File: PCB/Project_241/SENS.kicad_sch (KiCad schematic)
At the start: 15 parts, among them J2 Wind_Hall, J5 Rain_Hall, U3 LM393, U5 HDC1080

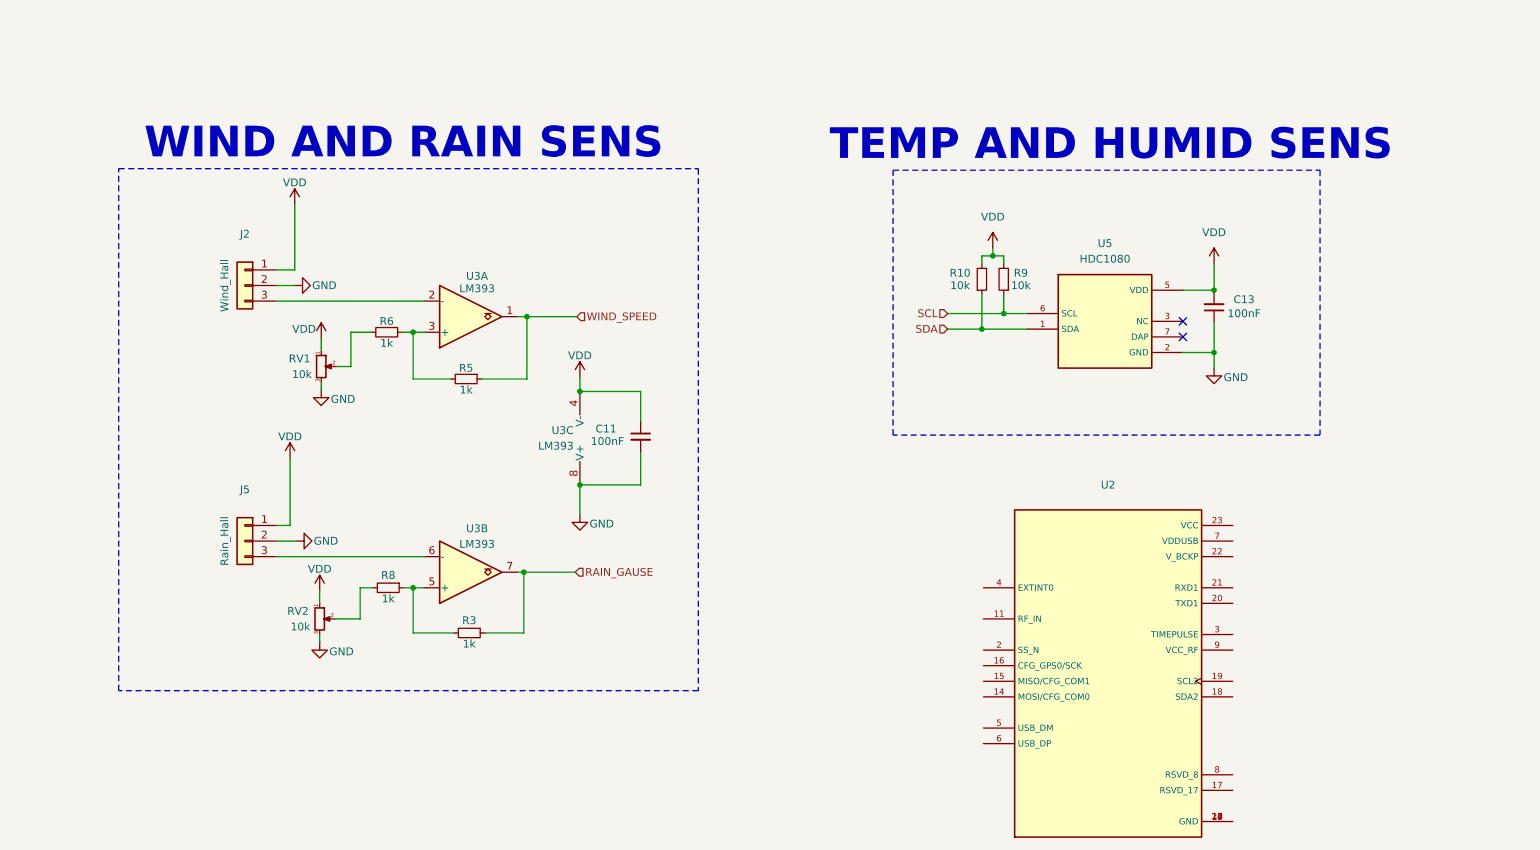
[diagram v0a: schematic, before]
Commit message: update gerber
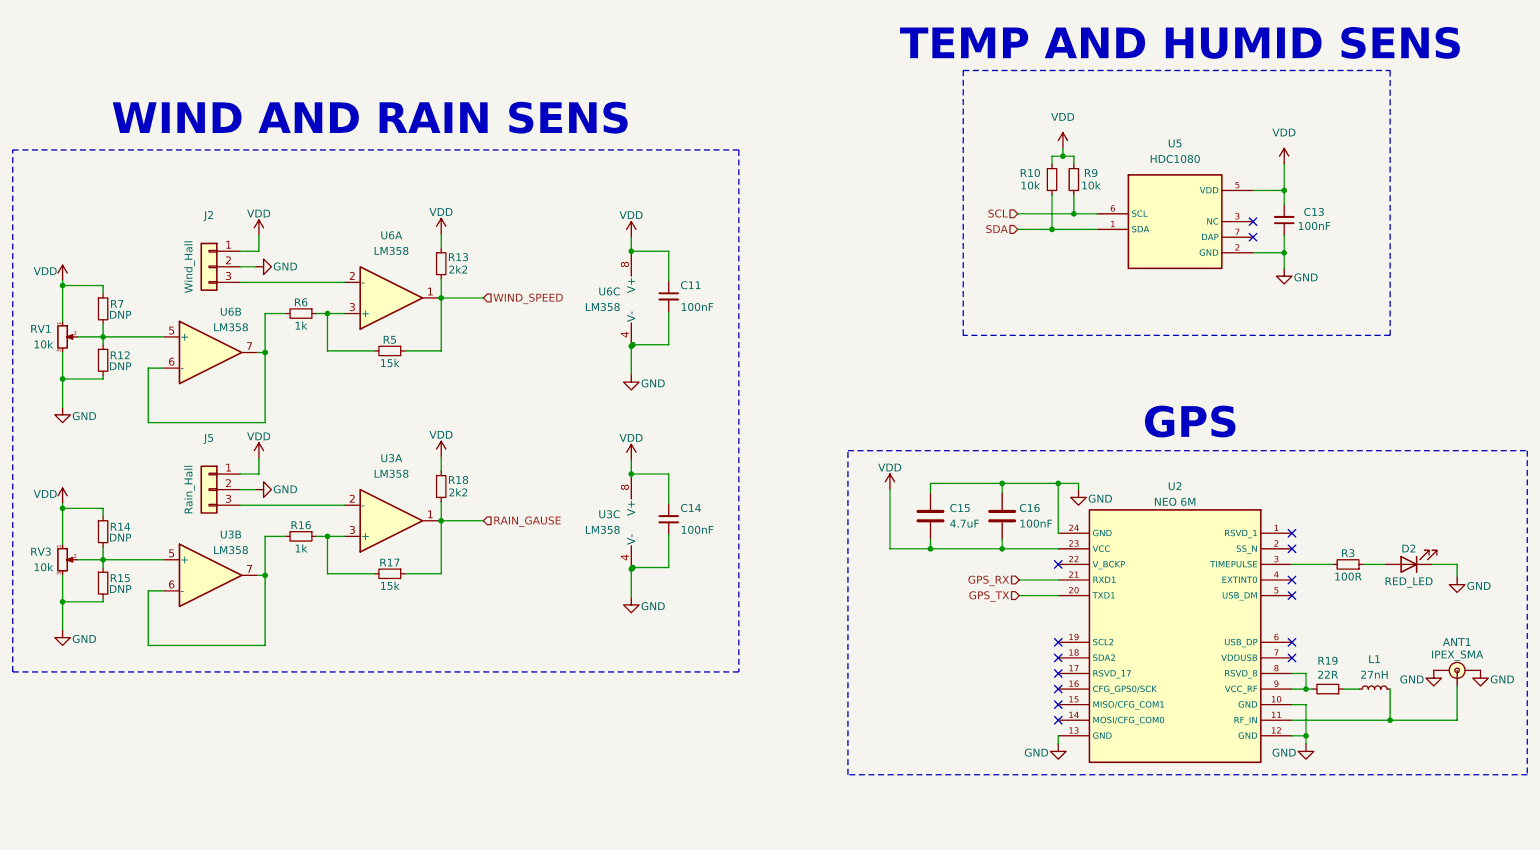
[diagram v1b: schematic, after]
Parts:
- removed R8: 1k, Resistor_SMD:R_0603_1608Metric, symbol Device:R_Small
- removed RV2: 10k, Resistor_SMD:R_0603_1608Metric, symbol Device:R_Potentiometer_Small
- removed U3: LM393, Package_SO:SO-8_3.9x4.9mm_P1.27mm, symbol Comparator:LM393
- added ANT1: IPEX_SMA, project241_footprint:ANT_SMA_3PIN, symbol project241_sym:IPEX_ANT
- added C14: 100nF, Capacitor_SMD:C_0603_1608Metric, symbol Device:C_Small
- added C15: 4.7uF, Capacitor_SMD:C_0603_1608Metric, symbol Device:C
- added C16: 100nF, Capacitor_SMD:C_0603_1608Metric, symbol Device:C
- added D2: RED_LED, LED_SMD:LED_0603_1608Metric, symbol Device:LED
- added L1: 27nH, Inductor_SMD:L_0603_1608Metric, symbol Device:L_Small
- added R12, R14, R15, R7: DNP, Resistor_SMD:R_0603_1608Metric, symbol Device:R_Small
- added R13, R18: 2k2, Resistor_SMD:R_0603_1608Metric, symbol Device:R_Small
- added R16: 1k, Resistor_SMD:R_0603_1608Metric, symbol Device:R_Small
- added R17: 15k, Resistor_SMD:R_0603_1608Metric, symbol Device:R_Small
- added R19: 22R, Resistor_SMD:R_0603_1608Metric, symbol Device:R_Small
- added RV3: 10k, project241_footprint:Poten_3PIN_SMD, symbol Device:R_Potentiometer_Small
- added U3, U6: LM358, IVSFootprint:SOIC-8, symbol Amplifier_Operational:LM358
- R3: value 1k -> 100R
- R5: value 1k -> 15k
- RV1: footprint Resistor_SMD:R_0603_1608Metric -> project241_footprint:Poten_3PIN_SMD
- U2: value ~ -> NEO 6M
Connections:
- net GND: now also U2.10 (GND), U2.12 (GND), U2.13 (GND), U2.24 (GND), ANT1.2 (GND), ANT1.3 (GND), C14.2, C15.1, C16.1, D2.1 (K), R12.2, R15.2, RV3.3, U3.4 (V-), U6.4 (V-)
- net RAIN_GAUSE: now also R17.1, R18.2, U3.1; no longer R3.1
- net VDD: now also U2.23 (VCC), C14.1, C15.2, C16.2, R13.1, R14.1, R18.1, R7.1, RV3.1, U3.8 (V+), U6.8 (V+)
- net WIND_SPEED: now also R13.2, U6.1
- net at R3.2: now also U2.3 (TIMEPULSE)
- net at J5.3 (Pin_3): now also U3.2 (-)
- net at R5.2, R6.1: now also U6.3 (+)
- net at R6.2: now also U6.6 (-), U6.7; no longer RV1.2
- net at J2.3 (Pin_3): now also U6.2 (-)
- net at U2.11 (RF_IN): now also ANT1.1 (FEED), L1.2
- net GPS_TX: now reaches U2.20 (TXD1)
- net GPS_RX: now reaches U2.21 (RXD1)
- net at U2.8 (RSVD_8): now also U2.9 (VCC_RF), R19.2
- new net: L1.1, R19.1
- new net: D2.2 (A), R3.1
- new net: R12.1, R7.2, RV1.2, U6.5 (+)
- new net: R16.1, R17.2, U3.3 (+)
- new net: R14.2, R15.1, RV3.2, U3.5 (+)
- new net: R16.2, U3.6 (-), U3.7
- no-connect marks 2 -> 15
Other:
- note added: "GPS"
- moved on the sheet: C11, C13, J2, J5, R10, R5, R6, R9, RV1, U5
